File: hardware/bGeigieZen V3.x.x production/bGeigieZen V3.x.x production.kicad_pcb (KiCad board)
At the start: 2 copper layers, 129.4 x 64.6 mm, 16 parts, among them J1 M5 2x15 pin, J10 QI GND, J11 QI charger Plus, J2 Geiger IRover, J3 GPS, J4 Geiger Safepulse, J5 Extra support header, J6 Grove, J8 QI charger ground, J9 QI Plus, SW1 SW_SPDT

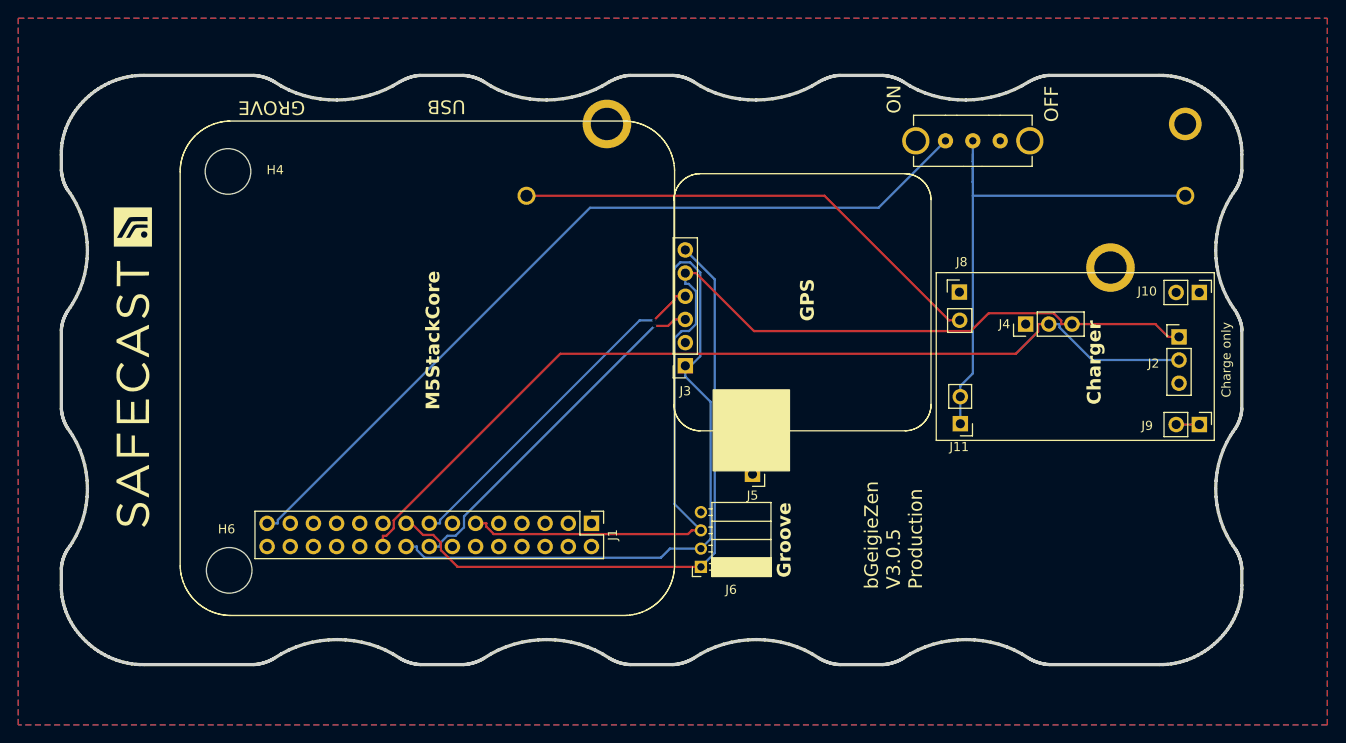
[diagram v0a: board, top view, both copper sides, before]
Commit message: Update Board V3.0.5
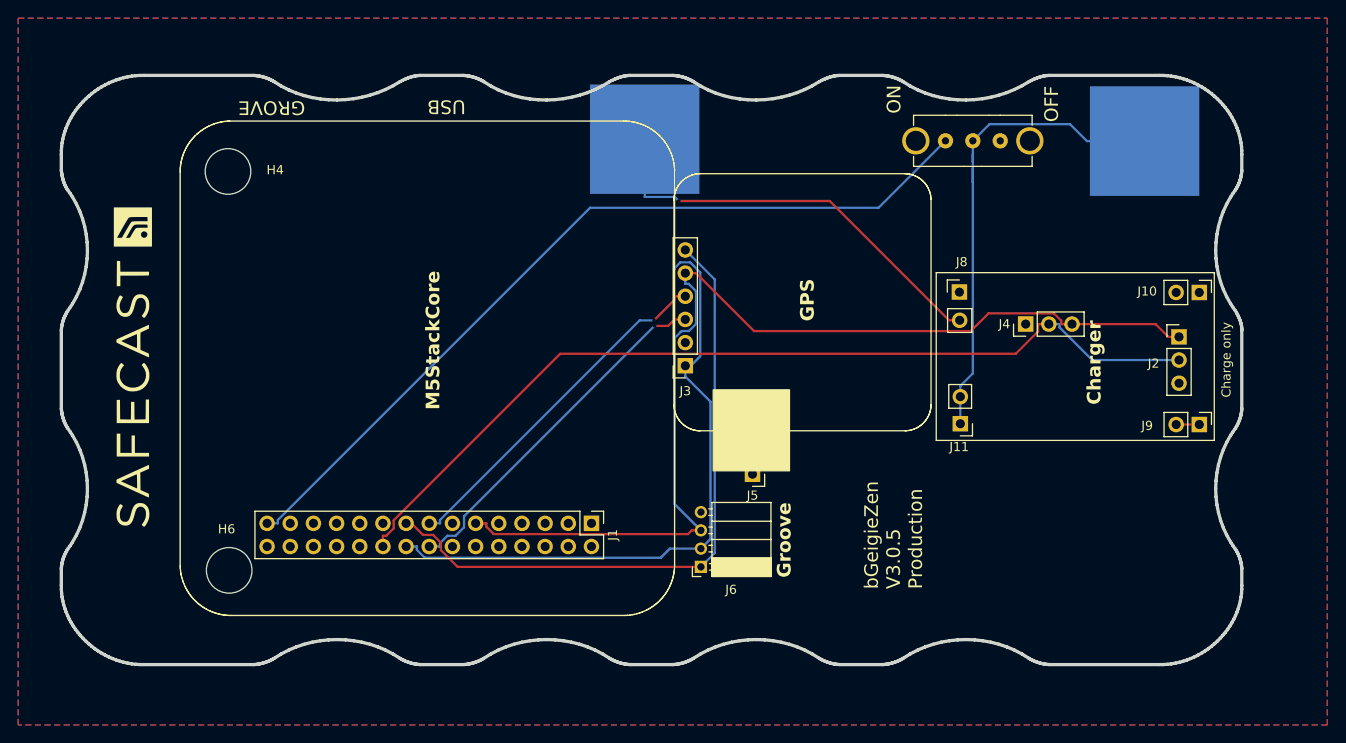
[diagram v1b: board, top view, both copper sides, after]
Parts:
- BT1: footprint bGeigieZen:1043 -> bGeigieZen:BATTERY_18650-HOLDER
- moved BT1 32.2 mm to (176.1, 73.9), turned to 180 degrees
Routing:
- net Net-(BT1--): track 53.1 -> 46.5 mm, vias 0 -> 1
- net /VBATT: track 57.1 -> 54.2 mm
